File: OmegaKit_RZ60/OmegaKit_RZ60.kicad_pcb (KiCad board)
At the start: 2 copper layers, 92.5 x 46 mm, 23 parts, among them SW1 SW_CK_OS102011MS2Q, U1 AMS1117-5.0

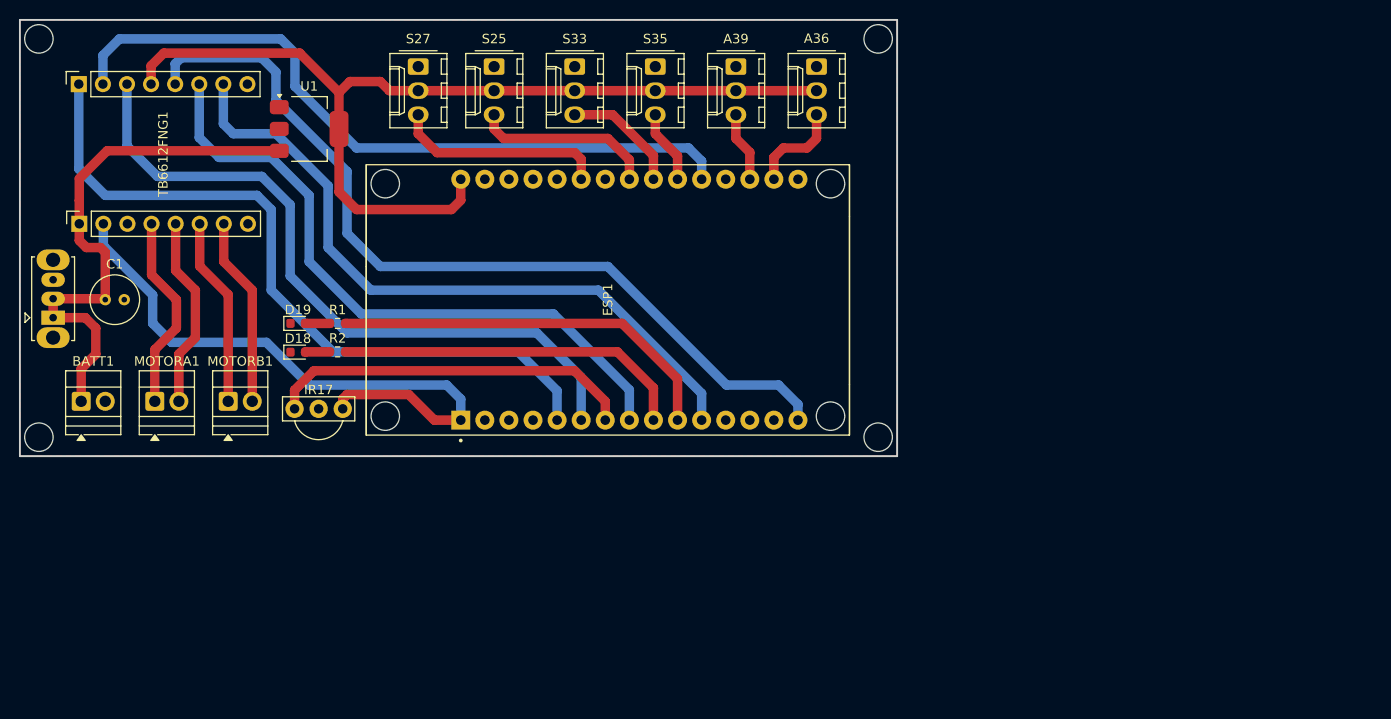
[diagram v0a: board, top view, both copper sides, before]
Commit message: Mudanças RZ60 + Placa juniores
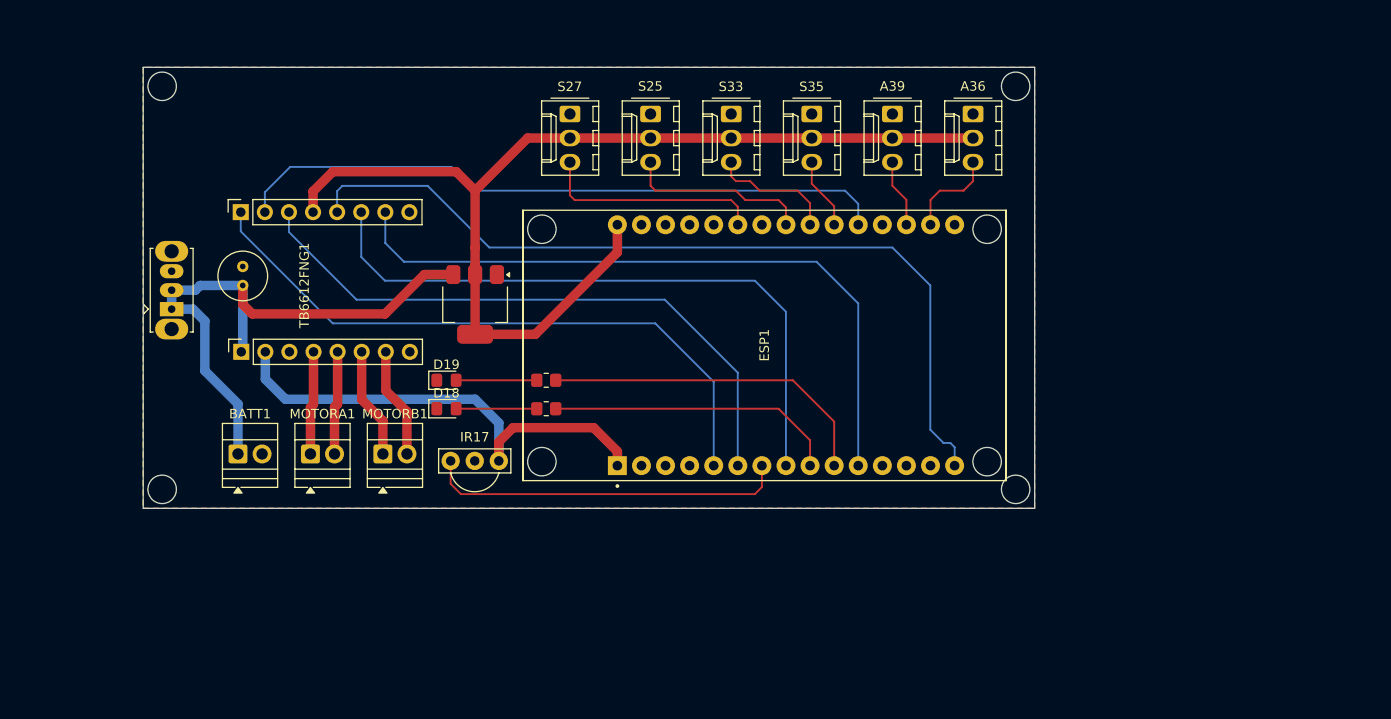
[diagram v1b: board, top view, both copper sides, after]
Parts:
- removed the ? at (136.0, 131.0)
- removed the ? at (224.5, 89.0)
- removed the ? at (136.0, 89.0)
- removed the ? at (224.5, 131.0)
- added ?: , , F.Cu at (239.0, 94.0)
- added ?: , , F.Cu at (149.0, 94.0)
- added ?: , , F.Cu at (149.0, 136.5)
- added ?: , , F.Cu at (239.0, 136.5)
- D18, D19: footprint LED_SMD:LED_0603_1608Metric -> LED_SMD:LED_0805_2012Metric_Pad1.15x1.40mm_HandSolder
- R1, R2: footprint Resistor_SMD:R_0603_1608Metric -> Resistor_SMD:R_0805_2012Metric_Pad1.20x1.40mm_HandSolder
- moved U1 25.5 mm to (182.0, 117.0), turned to -90 degrees
- moved R1 22.8 mm to (189.5, 125.0)
- moved R2 22.8 mm to (189.5, 128.0)
- moved TB6612FNG1 21.8 mm to (157.3, 122.0)
- moved BATT1 17.4 mm to (157.0, 132.8)
- moved IR17 17.4 mm to (182.0, 133.5)
- moved MOTORA1 17.3 mm to (164.6, 132.8)
- moved A36 17.2 mm to (234.5, 96.9)
- moved A39 17.2 mm to (226.0, 96.9)
- moved S25 17.2 mm to (200.5, 96.9)
- moved S33 17.2 mm to (209.0, 96.9)
- moved S35 17.2 mm to (217.5, 96.9)
- moved MOTORB1 17.2 mm to (172.3, 132.8)
- moved ESP1 17.2 mm to (212.5, 121.3)
- moved D19 16.8 mm to (179.0, 125.0)
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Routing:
- net /VCC: track 65.5 -> 51.1 mm
- net /V_REG: track 102.0 -> 113.4 mm
- net /A_VCC: track 20.7 -> 10.9 mm
- net /PWMA: track 77.1 -> 67.3 mm
- net /A_GND: track 20.3 -> 10.9 mm
- net /B_GND: track 20.0 -> 11.7 mm
- net /B_VCC: track 20.0 -> 11.7 mm
- net /AIN1: track 73.4 -> 65.4 mm
- net /AIN2: track 76.2 -> 69.6 mm
- net /LED2: track 37.5 -> 30.9 mm
- net /LED1: track 41.8 -> 35.8 mm
- net Net-(D19-A): track 2.57 -> 8.50 mm
- net Net-(D18-A): track 2.58 -> 8.50 mm
- net /BATT_VCC: track 57.7 -> 62.6 mm
- net /S4: track 22.4 -> 23.6 mm
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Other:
- board size 92.5 x 46 mm -> 94 x 46.5 mm

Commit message: ✨ feat: atualização de todos os arquivps faltantes
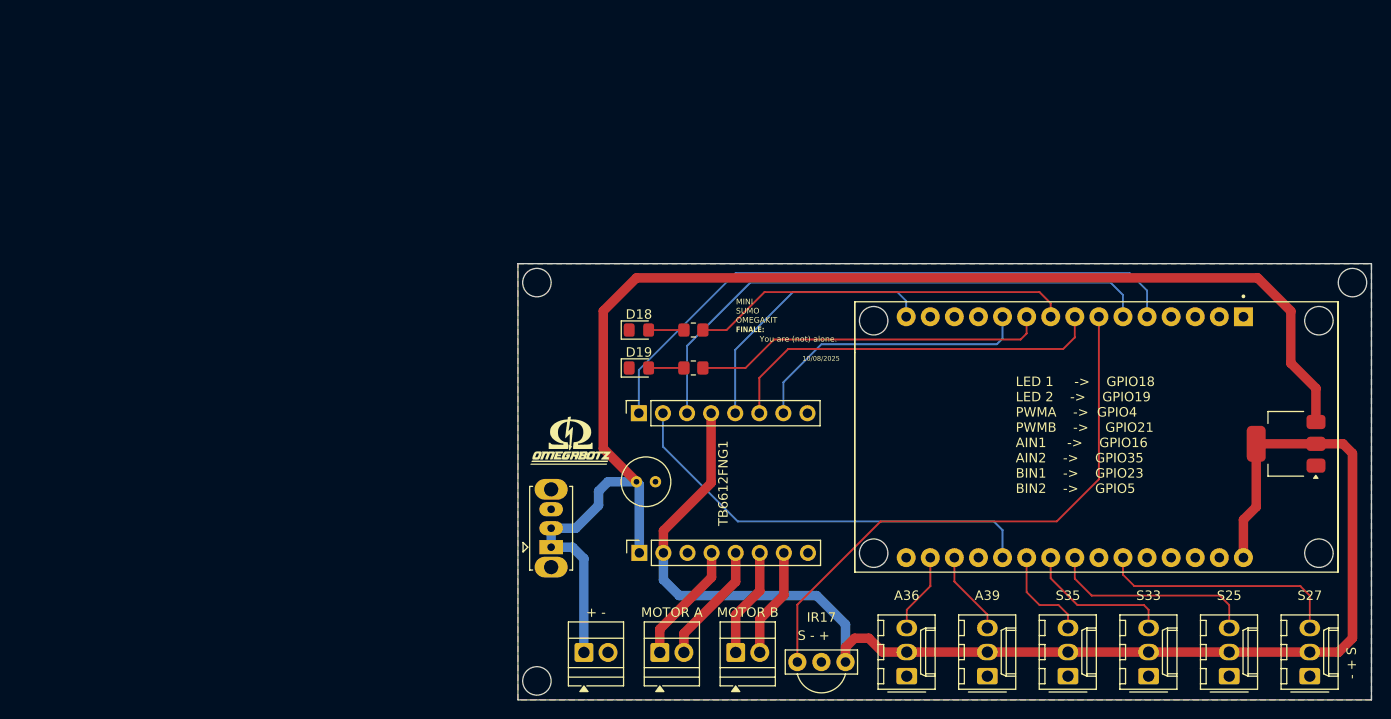
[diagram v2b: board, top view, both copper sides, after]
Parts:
- removed the ? at (239.0, 94.0)
- removed the ? at (149.0, 94.0)
- removed the ? at (149.0, 136.5)
- removed the ? at (239.0, 136.5)
- removed BATT1, MOTORA1, MOTORB1: Borne, TerminalBlock:TerminalBlock_Xinya_XY308-2.54-2P_1x02_P2.54mm_Horizontal
- added + -: Borne, TerminalBlock:TerminalBlock_Xinya_XY308-2.54-2P_1x02_P2.54mm_Horizontal, F.Cu at (193.5, 153.7)
- added ?: , , F.Cu at (188.5, 156.7)
- added ?: , , F.Cu at (188.5, 114.7)
- added ?: , , F.Cu at (274.5, 114.7)
- added MOTOR A: Borne, TerminalBlock:TerminalBlock_Xinya_XY308-2.54-2P_1x02_P2.54mm_Horizontal, F.Cu at (201.5, 153.7)
- added MOTOR B: Borne, TerminalBlock:TerminalBlock_Xinya_XY308-2.54-2P_1x02_P2.54mm_Horizontal, F.Cu at (209.5, 153.7)
- moved S27 98.0 mm to (270.0, 156.2), turned to 90 degrees
- moved U1 86.8 mm to (267.5, 131.7), turned to 180 degrees
- moved S25 85.1 mm to (261.5, 156.2), turned to 90 degrees
- moved S33 73.8 mm to (253.0, 156.2), turned to 90 degrees
- moved S35 65.1 mm to (244.5, 156.2), turned to 90 degrees
- moved A39 60.1 mm to (236.0, 156.2), turned to 90 degrees
- moved A36 59.7 mm to (227.5, 156.2), turned to 90 degrees
- moved SW1 47.2 mm to (190.0, 142.6)
- moved TB6612FNG1 47.0 mm to (199.3, 143.2)
- moved C1 46.4 mm to (199.0, 135.7), turned to 0 degrees
- moved IR17 42.3 mm to (218.5, 154.7)
- moved ESP1 36.3 mm to (247.5, 131.0), turned to -90 degrees
- moved D18 21.9 mm to (199.3, 119.7)
- moved D19 20.3 mm to (199.3, 123.7)
- moved R2 17.6 mm to (205.0, 119.7)
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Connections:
- IR17 pad 3: /VCC -> /V_REG
- TB6612FNG1 pad 2: /VCC -> /V_REG
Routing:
- net /BATT_VCC: track 62.6 -> 143.0 mm
- net /BIN1: track 89.8 -> 29.3 mm
- net /VCC: track 51.1 -> 0.00 mm
- net /PWMB: track 72.9 -> 30.6 mm
- net /V_REG: track 113.4 -> 144.0 mm
- net /BIN2: track 68.1 -> 40.9 mm
- net /AIN2: track 69.6 -> 45.9 mm
- net /IR_SIGNAL: track 38.3 -> 60.5 mm
- net /LED2: track 30.9 -> 40.2 mm
- net /AIN1: track 65.4 -> 58.7 mm
- net Net-(D19-A): track 8.50 -> 3.72 mm
- net Net-(D18-A): track 8.50 -> 3.72 mm
- net /S1: track 7.58 -> 10.4 mm
- net /S2: track 13.3 -> 15.8 mm
- net /S3: track 19.5 -> 22.1 mm
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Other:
- board size 94 x 46.5 mm -> 90 x 46 mm
- board text added: "- + S"
- board text added: "10/08/2025"
- board text added: "FINALE:"
- board text added: "LED 1 -> GPIO18 LED 2 -> GPIO19 PWMA -> GPIO4 PWMB -> GPIO21 AIN1 -> GPIO16 AIN2 -> GPIO35 BIN1 -> GPIO23 BIN2 -> GPIO5"
- board text added: "MINI SUMO OMEGAKIT"
- board text added: "S - +"
- board text added: "You are (not) alone."
